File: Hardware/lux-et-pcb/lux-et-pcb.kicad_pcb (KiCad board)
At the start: 2 copper layers, 80 x 54 mm, 87 parts, among them J1 Conn_01x03_Socket, J2 Conn_01x03_Socket, J3 Conn_01x03_Socket, J4 USB_C_Receptacle_PowerOnly_6P, Q1 PMOS, Q2 PMOS, Q3 AO3400A, Q4 AO3400A, Q5 AO3400A, Q7 2N7002K, U1 XL1509-5V, U2 AP2112K-3.3, U3 ESP32-WROOM-32, U4 TP4056

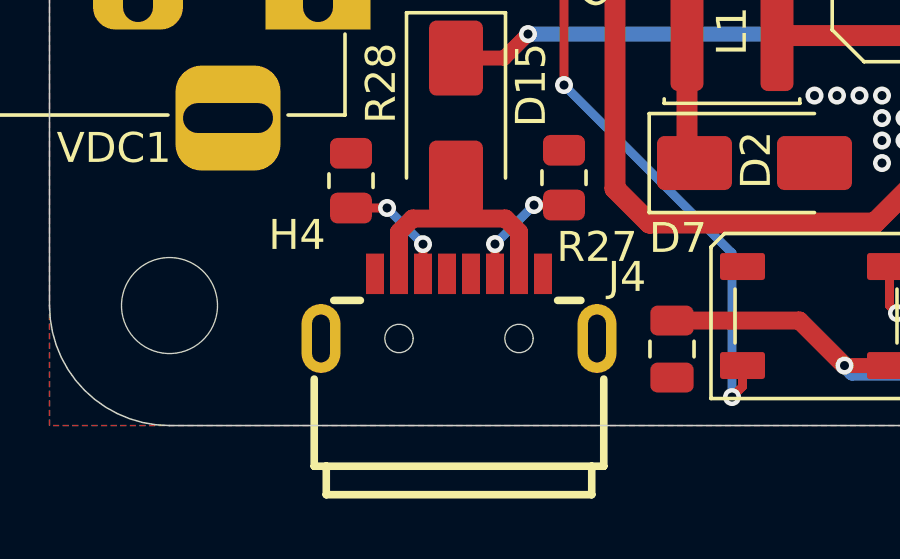
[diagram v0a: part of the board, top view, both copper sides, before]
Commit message: BoM update
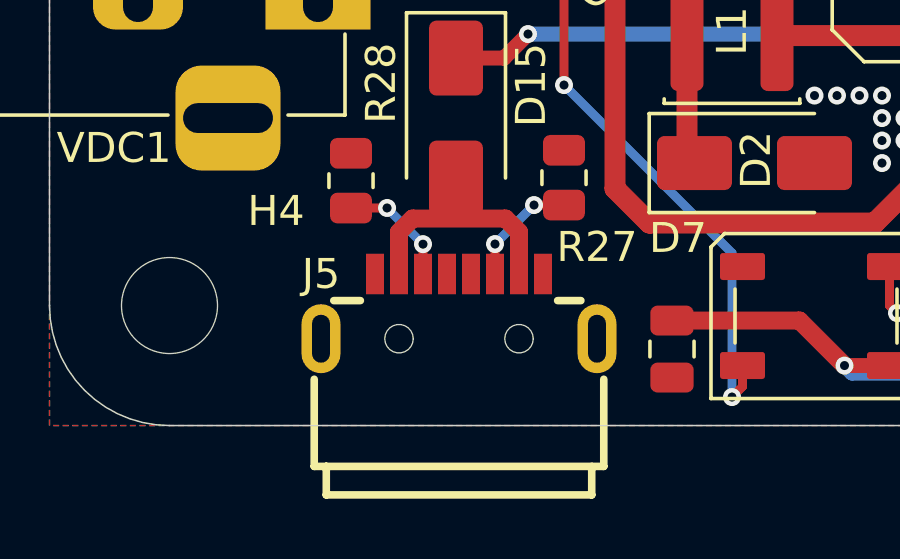
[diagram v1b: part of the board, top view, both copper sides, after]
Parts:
- removed J4: USB_C_Receptacle_PowerOnly_6P, Library:USB-C-SMD_GT-USB-7101A
- added J5: USB_C_Receptacle_USB2.0_8P, Library:USB-C-SMD_GT-USB-7101A, F.Cu at (133.4, 102.8)

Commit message: Hardware update
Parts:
- R11, R13, R17, R6: value 330 -> 330R
- R14, R15: value 1k -> 2.2k
- R18, R2, R3: value 2k2 -> 2.2k
- U5: value ~ -> XL4001
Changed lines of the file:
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@@
 			)
 		)
-		(property "Value" "1k"
+		(property "Value" "2.2k"
 			(at 0 1.65 90)
 			(layer "F.Fab")
@@
 			)
 		)
-		(property "LCSC" "C11702"
+		(property "LCSC" "C17520"
 			(at 0 0 -90)
 			(unlocked yes)
@@
 			)
 		)
-		(property "Sim.Pins" "1=D 2=G 3=S"
+		(property "Sim.Pins" "1=G 2=D 3=S"
 			(at 0 0 180)
 			(unlocked yes)
@@
 			)
 		)
-		(property "Value" "~"
+		(property "Value" "XL4001"
 			(at -0.325 4.2085 90)
 			(layer "F.Fab")
@@
 			)
 		)
-		(property "Value" "330"
+		(property "Value" "330R"
 			(at 0 1.65 90)
 			(layer "F.Fab")
@@
 			)
 		)
-		(property "Value" "330"
+		(property "Value" "330R"
 			(at 0 1.65 90)
 			(layer "F.Fab")
@@
 			)
 		)
-		(property "Value" "330"
+		(property "Value" "330R"
 			(at 0 1.65 90)
 			(layer "F.Fab")
@@
 			)
 		)
-		(property "Value" "2k2"
+		(property "Value" "2.2k"
 			(at 0 1.65 0)
 			(layer "F.Fab")
@@
 			)
 		)
-		(property "Value" "2k2"
+		(property "Value" "2.2k"
 			(at 0 1.65 90)
 			(layer "F.Fab")
@@
 			)
 		)
-		(property "Value" "1k"
+		(property "Value" "2.2k"
 			(at 0 1.65 90)
 			(layer "F.Fab")
@@
 			)
 		)
-		(property "LCSC" "C11702"
+		(property "LCSC" "C17520"
 			(at 0 0 -90)
 			(unlocked yes)
@@
 			)
 		)
-		(property "Value" "2k2"
+		(property "Value" "2.2k"
 			(at 0 1.65 90)
 			(layer "F.Fab")
@@
 			)
 		)
-		(property "Value" "330"
+		(property "Value" "330R"
 			(at 0 1.65 90)
 			(layer "F.Fab")
